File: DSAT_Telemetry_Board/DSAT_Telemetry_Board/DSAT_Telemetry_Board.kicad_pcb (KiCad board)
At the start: 4 copper layers, 152.7 x 108.5 mm, 96 parts, among them IC1 CG2409X3-C2, J1 Conn_01x04_Female, J2 Conn_Coaxial, J3 Conn_01x02_Female, J5 Conn_01x04_Male, SW1 SW_Push, SW2 SW_SPDT, U1 AMS1117-3.3, U2 AMS1117-3.3, U3 AMS1117-3.3, U4 AMS1117-3.3, U5 STM32L433RCTx, U6 Si4463, U7 PSA4-5043+, U8 Watchdog_Timer, Y1 16MHz, Y2 30MHz

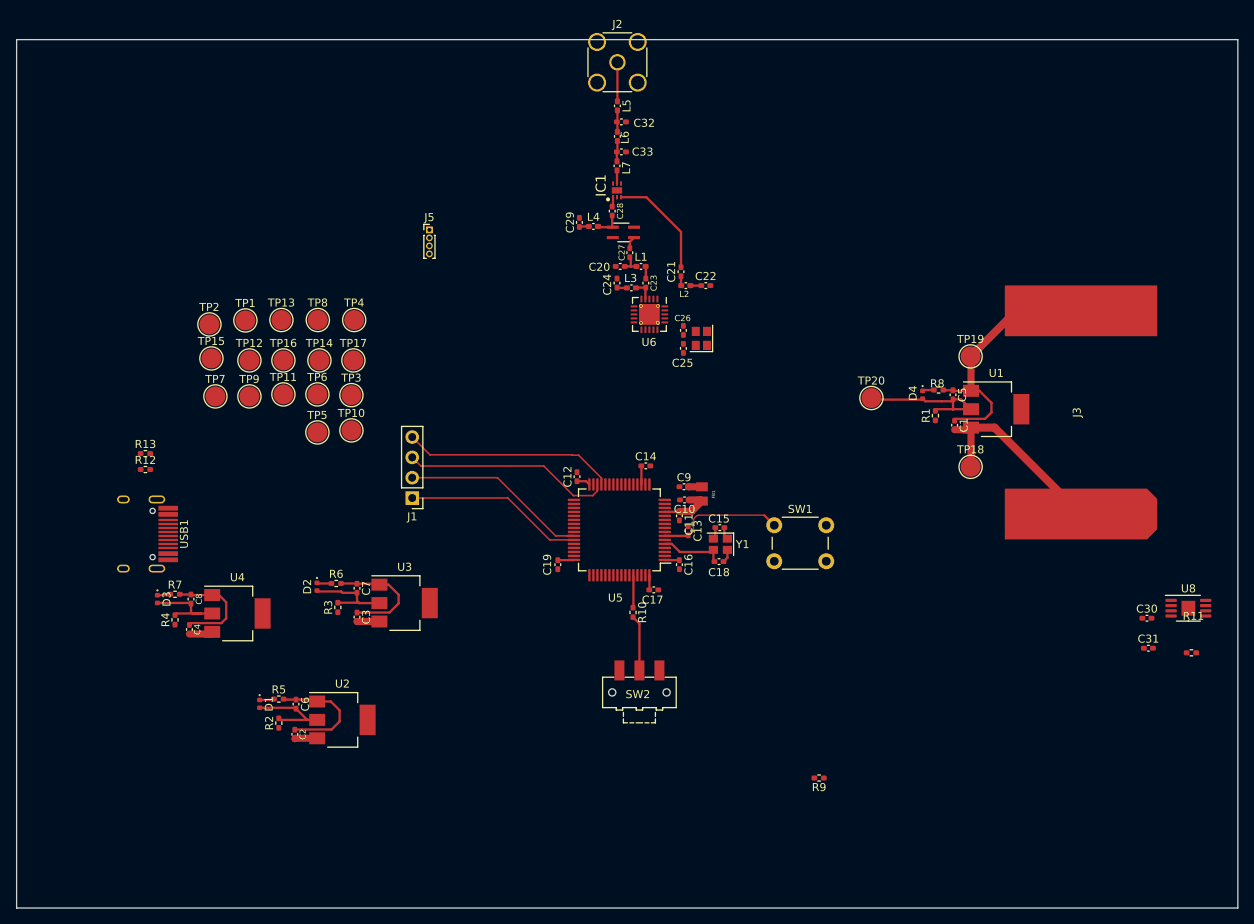
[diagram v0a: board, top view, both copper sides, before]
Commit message: Layout halfway done
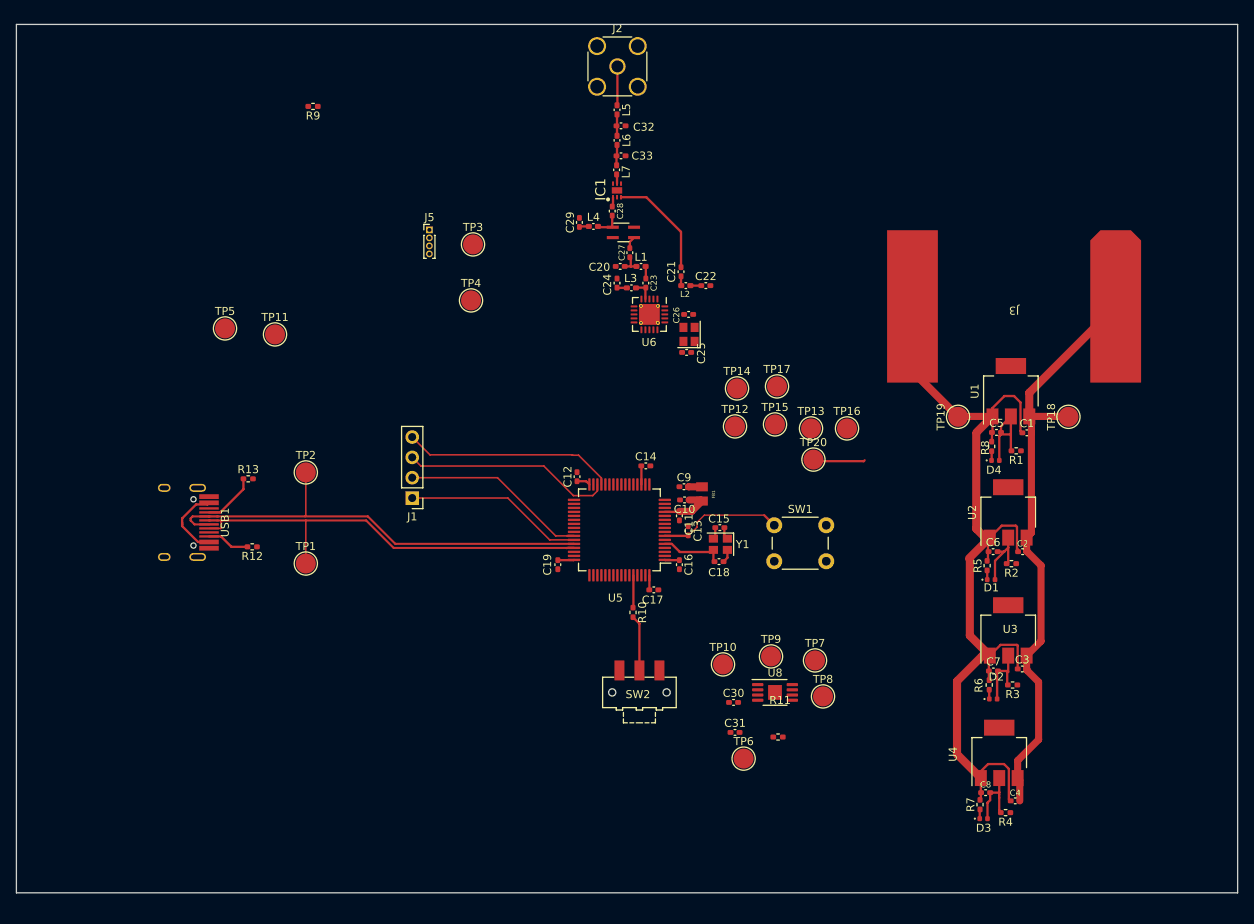
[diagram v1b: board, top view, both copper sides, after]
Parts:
- moved D3 106.9 mm to (249.8, 151.8), turned to 0 degrees
- moved R4 106.6 mm to (252.6, 151.0), turned to 180 degrees
- moved C4 105.4 mm to (253.8, 149.6), turned to 0 degrees
- moved R9 105.1 mm to (166.0, 62.8)
- moved R7 104.0 mm to (249.4, 150.0), turned to 90 degrees
- moved C8 102.2 mm to (250.1, 148.5), turned to 0 degrees
- moved U4 96.8 mm to (251.8, 143.6), turned to 90 degrees
- moved C2 93.8 mm to (254.7, 118.4), turned to 0 degrees
- moved R2 93.7 mm to (253.3, 119.9), turned to 180 degrees
- moved D1 92.7 mm to (250.8, 121.9), turned to 0 degrees
- moved R5 90.1 mm to (250.3, 120.2), turned to 90 degrees
- moved C6 89.2 mm to (251.0, 118.4), turned to 0 degrees
- moved U2 87.2 mm to (252.9, 113.5), turned to 90 degrees
- moved D2 85.7 mm to (251.0, 136.8), turned to 0 degrees
- moved R3 84.9 mm to (253.4, 135.1), turned to 180 degrees
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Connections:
- R9 pad 2: /Microcontroller/USB_D- -> /D-
- U5 pad 44: /Microcontroller/USB_D- -> /D-
- U5 pad 45: /Microcontroller/USB_D+ -> /D+
- USB1 pad 11: +3.3V -> VBUS
- USB1 pad 2: +3.3V -> VBUS
- USB1 pad 5: /Microcontroller/USB_D- -> /D-
- USB1 pad 6: /Microcontroller/USB_D+ -> /D+
- USB1 pad 7: /USBC to USB 2.2/USB_D- -> /D-
- USB1 pad 8: /USBC to USB 2.2/USB_D+ -> /D+
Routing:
- net /D-: track 0.00 -> 58.1 mm
- net /D+: track 0.00 -> 55.1 mm
- net VBUS: track 33.9 -> 84.9 mm
- net GND: track 79.8 -> 112.4 mm
- net Net-(R13-Pad1): track 0.00 -> 6.80 mm
- net Net-(R12-Pad2): track 0.00 -> 5.34 mm
- net Net-(C7-Pad2): track 11.7 -> 8.71 mm
- net Net-(C6-Pad2): track 11.5 -> 8.92 mm
- net Net-(C8-Pad2): track 11.0 -> 8.63 mm
- net Net-(C5-Pad2): track 18.6 -> 17.6 mm
- net /Microcontroller/NRST: track 14.8 -> 15.6 mm
- net Net-(D2-Pad1): track 1.84 -> 1.16 mm
- net Net-(D1-Pad1): track 1.85 -> 1.25 mm
- net Net-(D3-Pad1): track 1.81 -> 1.21 mm
- net Net-(D4-Pad1): track 1.32 -> 0.76 mm
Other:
- board size 152.7 x 108.5 mm -> 152.7 x 108.6 mm

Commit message: Layout changes
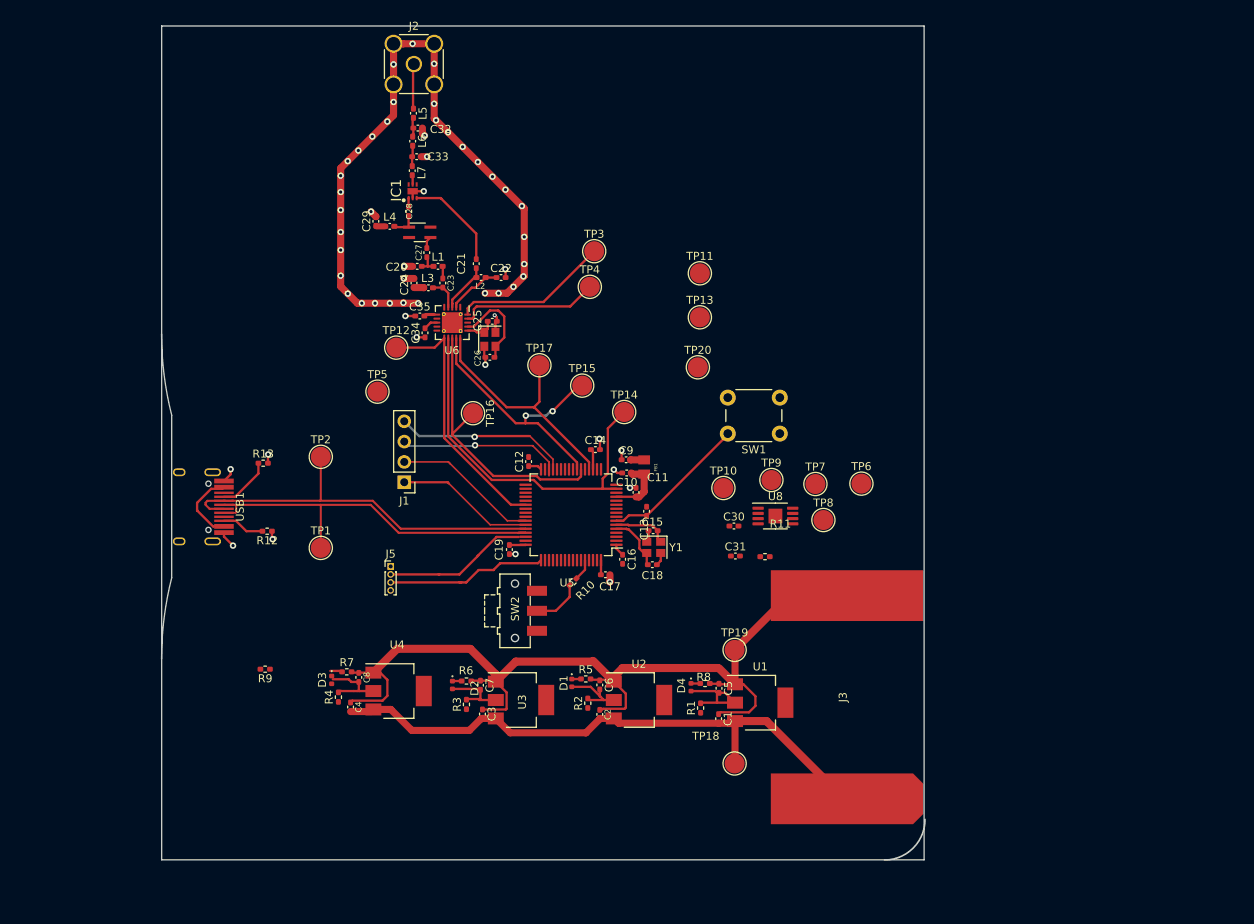
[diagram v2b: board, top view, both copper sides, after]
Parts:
- added C34: 100nF, Capacitor_SMD:C_0402_1005Metric_Pad0.74x0.62mm_HandSolder, F.Cu at (180.0, 91.0)
- added C35: 100nF, Capacitor_SMD:C_0402_1005Metric_Pad0.74x0.62mm_HandSolder, F.Cu at (179.3, 89.0)
- moved R4 84.6 mm to (169.2, 136.6), turned to 90 degrees
- moved C4 83.9 mm to (170.7, 137.8), turned to -90 degrees
- moved D3 83.3 mm to (168.3, 134.4), turned to -90 degrees
- moved R7 80.9 mm to (170.2, 133.4), turned to 0 degrees
- moved C8 79.7 mm to (171.7, 134.1), turned to -90 degrees
- moved U4 75.5 mm to (176.7, 135.8), turned to 0 degrees
- moved R9 70.6 mm to (160.0, 133.1)
- moved R3 68.3 mm to (185.2, 137.5), turned to 90 degrees
- moved C3 67.7 mm to (187.2, 138.7), turned to -90 degrees
- moved D2 67.6 mm to (183.4, 135.1), turned to -90 degrees
- moved R6 65.3 mm to (185.2, 134.6), turned to 0 degrees
- moved C7 64.1 mm to (186.9, 135.1), turned to -90 degrees
- moved U3 61.5 mm to (192.0, 136.9), turned to 0 degrees
- moved TP18 60.2 mm to (218.7, 144.9), turned to 0 degrees
- moved C2 56.6 mm to (201.8, 138.8), turned to -90 degrees
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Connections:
- U5 pad 15: /Microcontroller/TX_SCK -> /TX_SCLK
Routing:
- net GND: track 112.4 -> 224.9 mm, vias 0 -> 55
- net /TX_SCLK: track 0.00 -> 46.7 mm
- net /TX_SDO: track 0.00 -> 35.2 mm
- net /TX_SDI: track 0.00 -> 33.9 mm, vias 0 -> 2
- net /TX_~{IRQ}: track 0.00 -> 32.6 mm
- net /TX_~{SEL}: track 0.00 -> 29.9 mm
- net /Microcontroller/DEBUG_CLK: track 0.00 -> 20.3 mm
- net /TX_En: track 0.00 -> 19.6 mm
- net /Microcontroller/DEBUG_DIO: track 0.00 -> 18.2 mm
- net /RX_En: track 0.00 -> 17.5 mm
- net Net-(C26-Pad1): track 0.00 -> 11.3 mm
- net /D+: track 55.1 -> 47.2 mm
- net /D-: track 58.1 -> 50.2 mm
- net Net-(C5-Pad2): track 17.6 -> 11.6 mm
- net Net-(C22-Pad1): track 1.36 -> 6.86 mm
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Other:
- board size 152.7 x 108.6 mm -> 95.4 x 104.3 mm
